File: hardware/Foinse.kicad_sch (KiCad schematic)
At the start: 72 parts, among them J1 ESQ-110-X-X-D, J2 XT30PW-M, J4 PJ-002AH, J6 JTAG-10 PIN, U1 STM32F072C8Tx, U15 INA239AIDGSR, U16 INA239AIDGSR, U17 LTC4412xS6, U19 TPS56A37RPAR, U2 TLV70433DBVT, U4 TJA1051T-3, U5 TPS563203

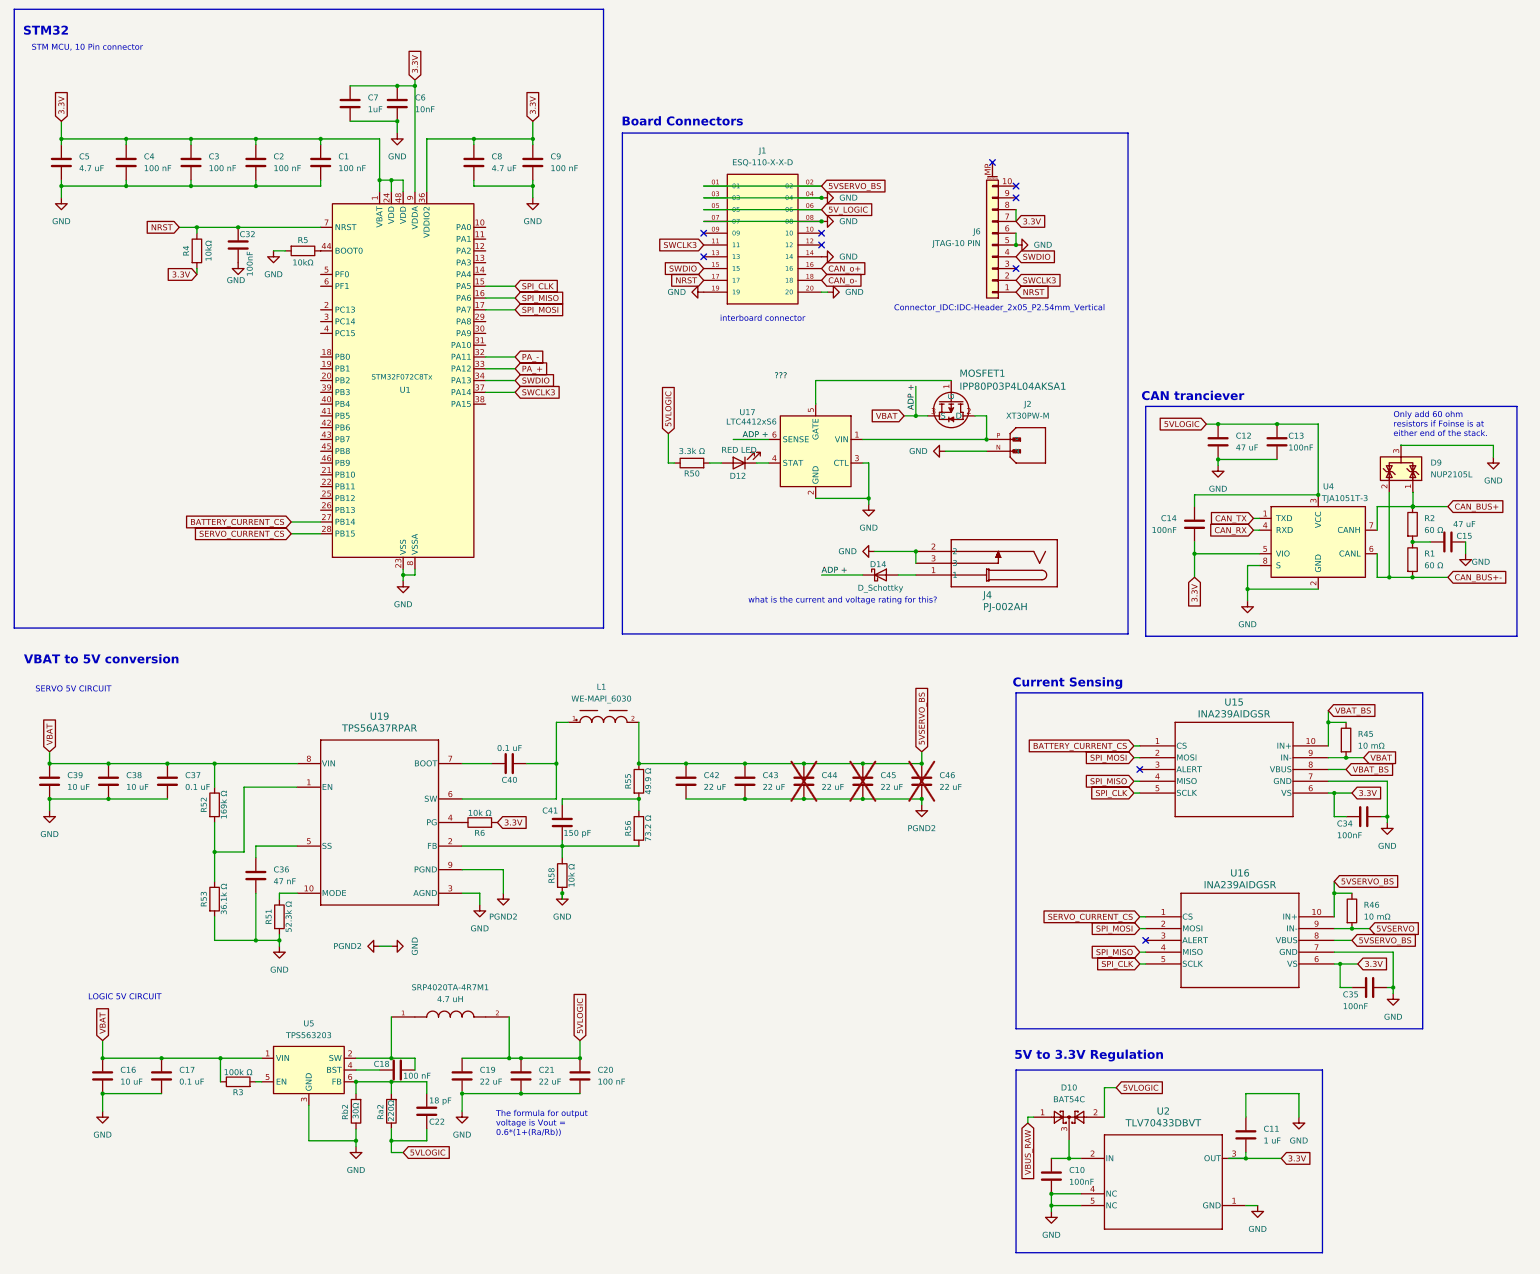
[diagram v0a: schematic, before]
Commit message: gonna
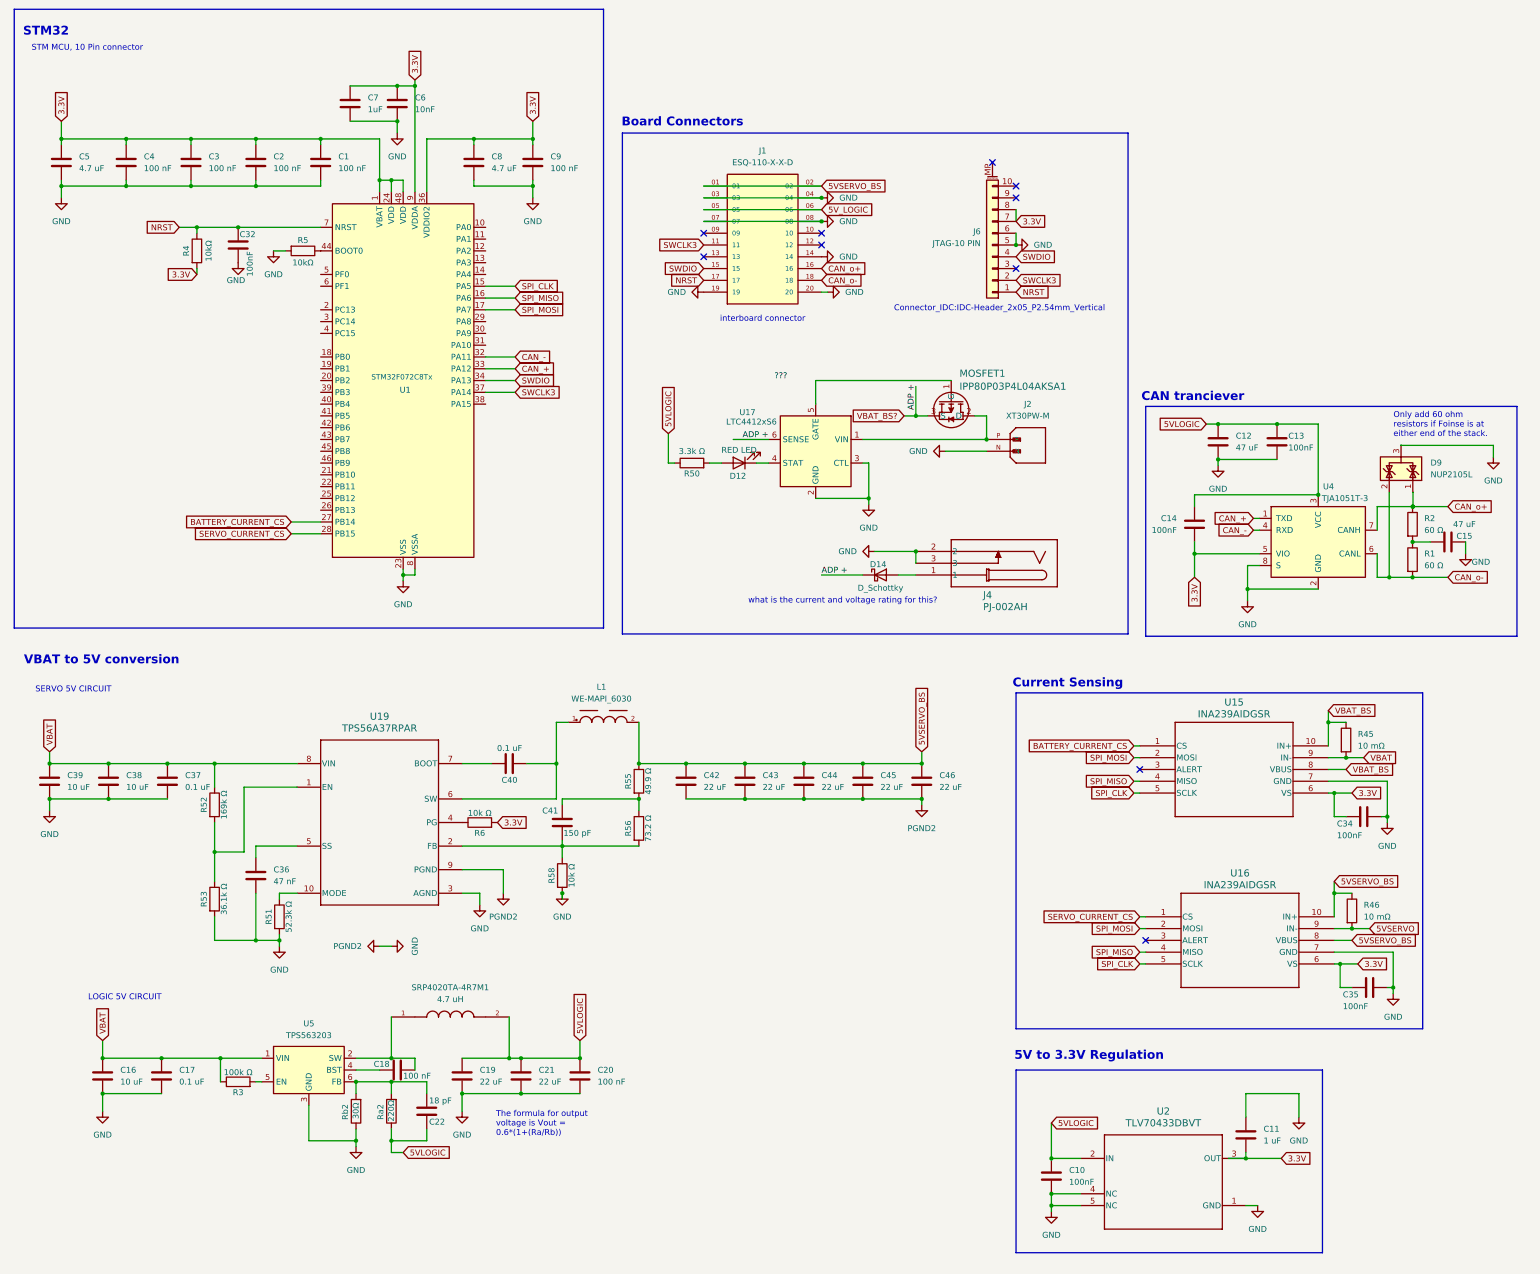
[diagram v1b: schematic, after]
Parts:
- removed D10: BAT54C, Package_TO_SOT_SMD:SOT-23, symbol Diode:BAT54C
- C44, C45, C46: now fitted
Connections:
- net CAN_BUS+ is gone; now on net CAN_o+: D9.1 (K), R2.1, U4.7 (CANH)
- net CAN_BUS+- is gone; now on net CAN_o-: D9.2 (K), R1.2, U4.6 (CANL)
- net PA_+ is gone; now on net CAN_+: U1.33 (PA12)
- net PA_- is gone; now on net CAN_-: U1.32 (PA11)
- net 5VLOGIC: now also C10.1, U2.2 (IN)
- net VBAT: no longer D14.1 (K), MOSFET1.3 (S), U17.6 (SENSE)
- net CAN_RX renamed CAN_-
- net CAN_TX renamed CAN_+
- new net VBAT_BS?: D14.1 (K), MOSFET1.3 (S), U17.6 (SENSE)
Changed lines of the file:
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@@
 	)
 	(junction
+		(at 336.55 322.58)
+		(diameter 0)
+		(color 0 0 0 0)
+	)
+	(junction
 		(at 231.14 265.43)
 		(diameter 0)
@@
 	)
 	(junction
-		(at 340.36 322.58)
-		(diameter 0)
-		(color 0 0 0 0)
-	)
-	(junction
 		(at 408.94 248.92)
 		(diameter 0)
@@
 	(wire
 		(pts
-			(xy 340.36 322.58) (xy 342.9 322.58)
-		)
-		(stroke
-			(width 0)
-			(type default)
-		)
-	)
-	(wire
-		(pts
 			(xy 410.21 278.13) (xy 410.21 285.75)
 		)
@@
 	(wire
 		(pts
-			(xy 331.47 313.69) (xy 331.47 314.96)
-		)
-		(stroke
-			(width 0)
-			(type default)
-		)
-	)
-	(wire
-		(pts
 			(xy 231.14 254) (xy 231.14 255.27)
 		)
@@
 	(wire
 		(pts
-			(xy 347.98 313.69) (xy 347.98 307.34)
-		)
-		(stroke
-			(width 0)
-			(type default)
-		)
-	)
-	(wire
-		(pts
 			(xy 231.14 255.27) (xy 231.14 257.81)
 		)
@@
 	(wire
 		(pts
-			(xy 347.98 307.34) (xy 350.52 307.34)
-		)
-		(stroke
-			(width 0)
-			(type default)
-		)
-	)
-	(wire
-		(pts
 			(xy 224.79 102.87) (xy 224.79 104.14)
 		)
@@
 	(wire
 		(pts
-			(xy 340.36 318.77) (xy 340.36 322.58)
+			(xy 336.55 314.96) (xy 336.55 322.58)
 		)
 		(stroke
@@
 	(wire
 		(pts
-			(xy 332.74 313.69) (xy 331.47 313.69)
-		)
-		(stroke
-			(width 0)
-			(type default)
-		)
-	)
-	(wire
-		(pts
 			(xy 196.85 196.85) (xy 196.85 198.12)
 		)
@@
 	(wire
 		(pts
-			(xy 336.55 322.58) (xy 340.36 322.58)
+			(xy 336.55 322.58) (xy 342.9 322.58)
 		)
 		(stroke
@@
 	(global_label "5VLOGIC"
 		(shape input)
-		(at 350.52 307.34 0)
+		(at 336.55 314.96 0)
 		(fields_autoplaced yes)
 		(effects
@@
 		)
 		(property "Intersheetrefs" "${INTERSHEET_REFS}"
-			(at 361.3067 307.34 0)
+			(at 347.3367 314.96 0)
 			(effects
 				(font
@@
 		)
 	)
-	(global_label "PA_-"
+	(global_label "CAN_-"
 		(shape input)
 		(at 220.98 149.86 0)
@@
 		)
 		(property "Intersheetrefs" "${INTERSHEET_REFS}"
-			(at 228.8638 149.86 0)
+			(at 230.1943 149.86 0)
 			(effects
 				(font
@@
 		)
 	)
-	(global_label "CAN_BUS+"
+	(global_label "CAN_o+"
 		(shape input)
 		(at 422.003 182.1073 0)
@@
 		)
 		(property "Intersheetrefs" "${INTERSHEET_REFS}"
-			(at 435.0273 182.1073 0)
+			(at 432.3663 182.1073 0)
 			(effects
 				(font
@@
 		)
 	)
-	(global_label "CAN_TX"
+	(global_label "CAN_+"
 		(shape input)
 		(at 380.093 184.6473 180)
@@
 		)
 		(property "Intersheetrefs" "${INTERSHEET_REFS}"
-			(at 370.274 184.6473 0)
+			(at 370.8787 184.6473 0)
 			(effects
 				(font
@@
 		)
 	)
-	(global_label "VBAT"
+	(global_label "VBAT_BS?"
 		(shape input)
 		(at 304.8 162.56 180)
@@
 		)
 		(property "Intersheetrefs" "${INTERSHEET_REFS}"
-			(at 297.4 162.56 0)
+			(at 292.8643 162.56 0)
 			(effects
 				(font
@@
 		)
 	)
-	(global_label "VBUS_RAW"
-		(shape input)
-		(at 331.47 314.96 270)
-		(fields_autoplaced yes)
-		(effects
-			(font
-				(size 1.27 1.27)
-			)
-			(justify right)
-		)
-		(property "Intersheetrefs" "${INTERSHEET_REFS}"
-			(at 331.47 327.6214 90)
-			(effects
-				(font
-					(size 1.27 1.27)
-				)
-				(justify right)
-				(hide yes)
-			)
-		)
-	)
 	(global_label "NRST"
 		(shape input)
@@
 		)
 	)
-	(global_label "CAN_RX"
+	(global_label "CAN_-"
 		(shape input)
 		(at 380.093 187.1873 180)
@@
 		)
 		(property "Intersheetrefs" "${INTERSHEET_REFS}"
-			(at 369.9716 187.1873 0)
+			(at 370.8787 187.1873 0)
 			(effects
 				(font
@@
 		)
 	)
-	(global_label "CAN_BUS+-"
+	(global_label "CAN_o-"
 		(shape input)
 		(at 422.003 197.3473 0)
@@
 		)
 		(property "Intersheetrefs" "${INTERSHEET_REFS}"
-			(at 436.5997 197.3473 0)
+			(at 432.3663 197.3473 0)
 			(effects
 				(font
@@
 		)
 	)
-	(global_label "PA_+"
+	(global_label "CAN_+"
 		(shape input)
 		(at 220.98 152.4 0)
@@
 		)
 		(property "Intersheetrefs" "${INTERSHEET_REFS}"
-			(at 228.8638 152.4 0)
+			(at 230.1943 152.4 0)
 			(effects
 				(font
@@
 	)
 	(symbol
-		(lib_id "Diode:BAT54C")
-		(at 340.36 313.69 0)
-		(unit 1)
-		(exclude_from_sim no)
-		(in_bom yes)
-		(on_board yes)
-		(dnp no)
-		(fields_autoplaced yes)
-		(property "Reference" "D10"
-			(at 340.36 307.34 0)
-			(effects
-				(font
-					(size 1.27 1.27)
-				)
-			)
-		)
-		(property "Value" "BAT54C"
-			(at 340.36 309.88 0)
-			(effects
-				(font
-					(size 1.27 1.27)
-				)
-			)
-		)
-		(property "Footprint" "Package_TO_SOT_SMD:SOT-23"
-			(at 342.265 310.515 0)
-			(effects
-				(font
-					(size 1.27 1.27)
-				)
-				(justify left)
-				(hide yes)
-			)
-		)
-		(property "Datasheet" "http://www.diodes.com/_files/datasheets/ds11005.pdf"
-			(at 338.328 313.69 0)
-			(effects
-				(font
-					(size 1.27 1.27)
-				)
-				(hide yes)
-			)
-		)
-		(property "Description" "dual schottky barrier diode, common cathode"
-			(at 340.36 313.69 0)
-			(effects
-				(font
-					(size 1.27 1.27)
-				)
-				(hide yes)
-			)
-		)
-		(pin "1"
-		)
-		(pin "3"
-		)
-		(pin "2"
-		)
-		(instances
-			(project ""
-				(path "/e25e400c-9bc4-4e0b-8f6d-7db79788ea60"
-					(reference "D10")
-					(unit 1)
-				)
-			)
-		)
-	)
-	(symbol
 		(lib_id "power:GND")
 		(at 328.93 125.73 90)
@@
 		(in_bom yes)
 		(on_board yes)
-		(dnp yes)
+		(dnp no)
 		(property "Reference" "C46"
 			(at 312.42 240.03 0)
@@
 		(in_bom yes)
 		(on_board yes)
-		(dnp yes)
+		(dnp no)
 		(property "Reference" "C44"
 			(at 287.02 240.03 0)
@@
 		(in_bom yes)
 		(on_board yes)
-		(dnp yes)
+		(dnp no)
 		(property "Reference" "C45"
 			(at 299.72 240.03 0)

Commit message: give
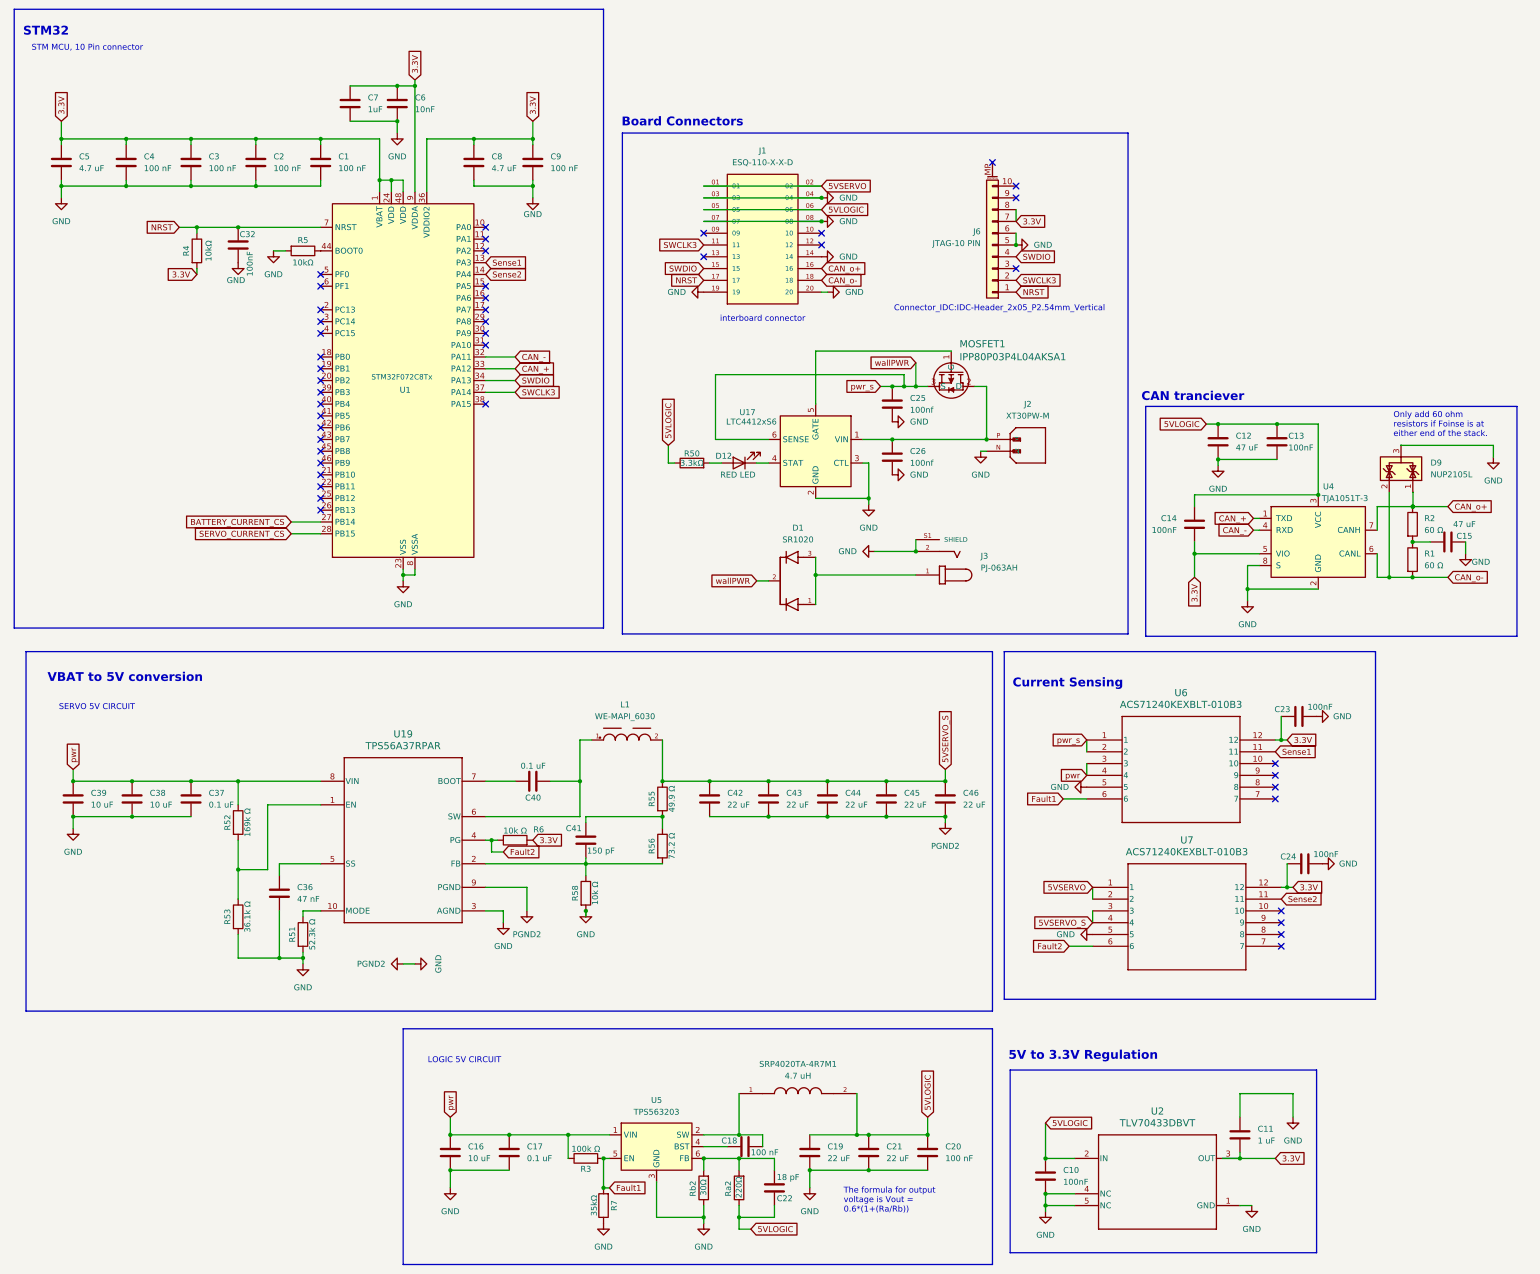
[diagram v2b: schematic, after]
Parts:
- removed C34, C35: 100nF, Capacitor_SMD:C_0402_1005Metric, symbol Device:C
- removed D14: D_Schottky, Package_TO_SOT_THT:TO-220-3_Vertical, symbol Device:D_Schottky
- removed J4: PJ-002AH, Foinse Footprints:PJ-002AH_CUD, symbol PJ-002AH:PJ-002AH
- removed R45, R46: 10 mΩ, Resistor_SMD:R_0402_1005Metric, symbol Device:R
- removed U15, U16: INA239AIDGSR, Foinse Footprints:VSSOP_9AIDGST_TEX, symbol INA239:INA239AIDGSR
- added C23, C24: 100nF, Capacitor_SMD:C_0402_1005Metric, symbol Device:C
- added C25, C26: 100nf, Capacitor_SMD:C_0402_1005Metric, symbol Device:C
- added D1: SR1020, footprints:TO254P1050X476X2020-3, symbol SR1020:SR1020
- added J3: PJ-063AH, footprints:CUI_PJ-063AH, symbol PJ-063AH:PJ-063AH
- added R7: 35kΩ, Resistor_SMD:R_0402_1005Metric, symbol Device:R
- added U6, U7: ACS71240KEXBLT-010B3, QFN12_ACS711KEXLT-31AB-T_ALM, symbol ACS71240KEXBLT:ACS71240KEXBLT-030B3
- R50: value 3.3k Ω -> 3.3kΩ
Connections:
- net 5V_LOGIC is gone; now on net 5VLOGIC: J1.05, J1.06
- net 3.3V: now also C23.2, C24.2, U6.12, U7.12
- net 5VSERVO: now also J1.01, J1.02, U7.1, U7.2
- net GND: now also C23.1, C24.1, C25.2, C26.2, J3.2, J3.S1 (SHIELD), J3.S2 (SHIELD), R7.1, U6.5, U7.5
- net at J2.P, MOSFET1.2 (D), U17.1 (VIN): now also C26.1
- net Fault2: now reaches R6.1, U19.4 (PG)
- net Fault2: now also U7.6
- net Fault1: now reaches R3.2, U5.5 (EN)
- net Fault1: now also R7.2, U6.6
- net Sense1: now reaches U1.13 (PA3)
- net Sense1: now also U6.11
- net Sense2: now reaches U1.14 (PA4)
- net Sense2: now also U7.11
- net 5VSERVO_BS renamed 5VSERVO_S
- net 5VSERVO_S: now also U7.3, U7.4; no longer J1.01, J1.02
- net SPI_CLK: no longer names the net of U1.15 (PA5)
- net SPI_MISO: no longer names the net of U1.16 (PA6)
- net SPI_MOSI: no longer names the net of U1.17 (PA7)
- net VBAT renamed pwr
- net pwr: now also U6.3, U6.4
- net VBAT_BS? renamed pwr_s
- net pwr_s: now also C25.1, D1.2, U6.1, U6.2
- new net: D1.1, D1.3, J3.1
- no-connect marks 10 -> 45
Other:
- note removed: "what is the current and voltage rating for this?"
- moved on the sheet: C10, C11, C16, C17, C18, C19, C20, C21, C22, C36, C37, C38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
